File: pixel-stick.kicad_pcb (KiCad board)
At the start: 2 copper layers, 16.5 x 37.1 mm, 16 parts, among them J2 WS28**, U1 AZ1117-3.3, U2 ESP-01v090, U3 SN74LVC1T45DBV, U4 RT9361A

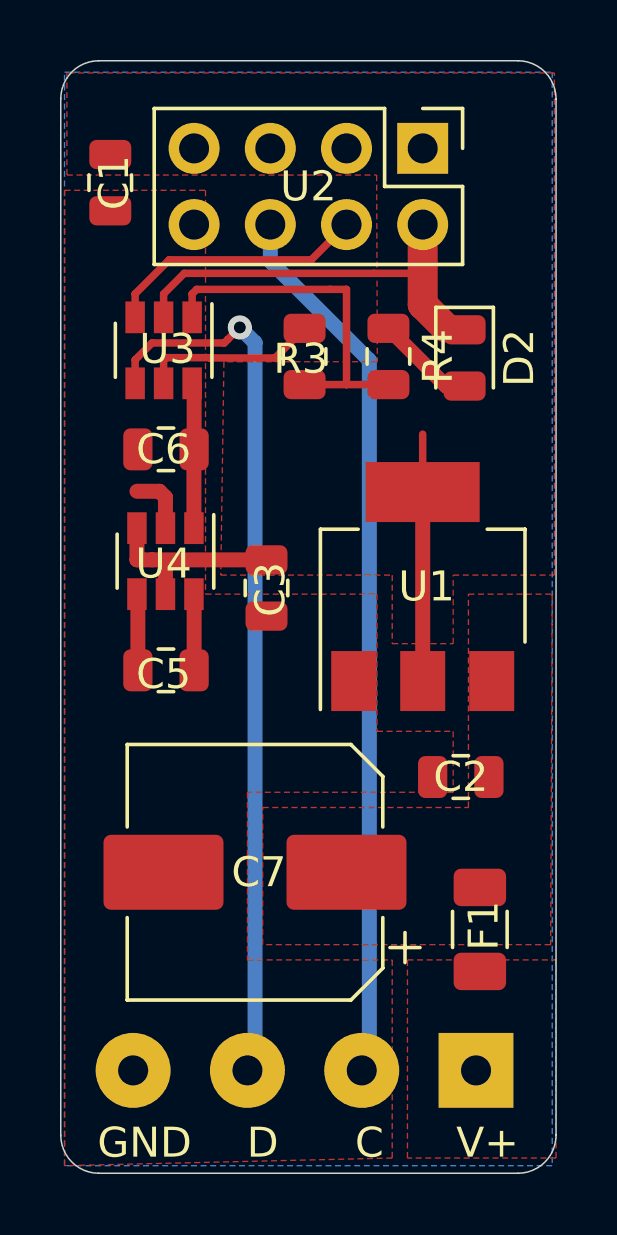
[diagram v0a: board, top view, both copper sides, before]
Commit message: fix drc errors
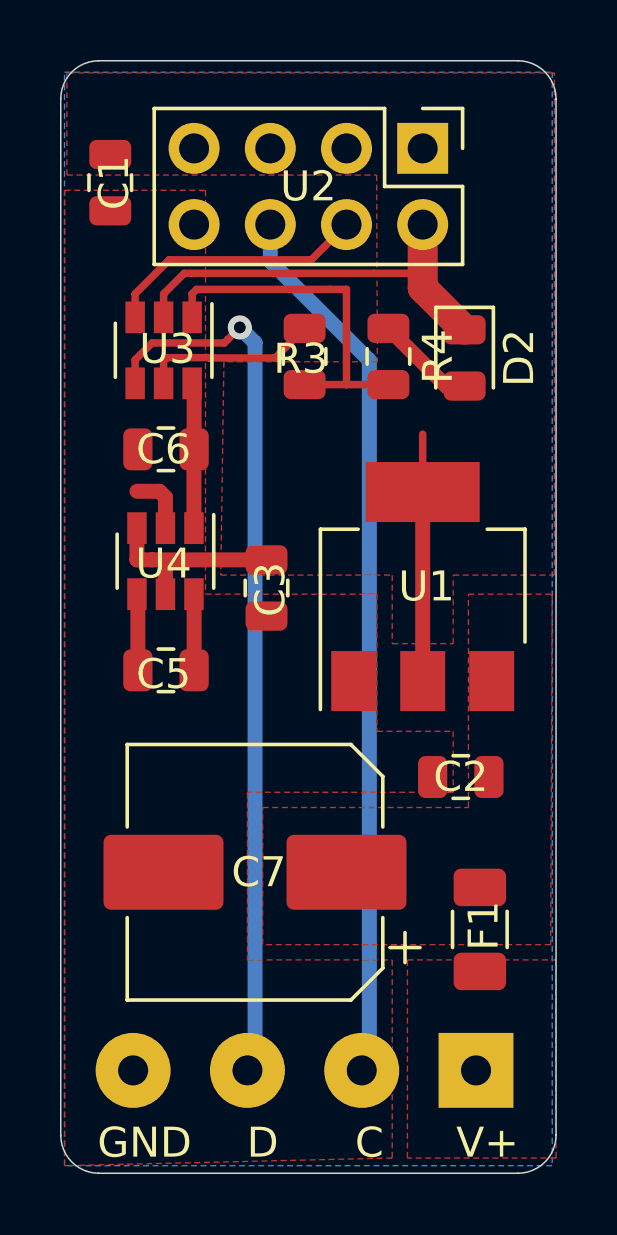
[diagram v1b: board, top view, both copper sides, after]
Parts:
- R4: value 10k -> 120
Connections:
- J2 pad 2: /DATA -> /CLOCK
- J2 pad 3: /CLOCK -> /DATA
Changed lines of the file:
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@@
   )
   (setup
-    (last_trace_width 0.25)
+    (last_trace_width 1)
     (user_trace_width 0.5)
     (user_trace_width 1)
@@
       (effects (font (size 1 1) (thickness 0.15)))
     )
-    (fp_text value 10k (at 0 1.65 90) (layer F.Fab)
+    (fp_text value 120 (at 0 1.65 90) (layer F.Fab)
       (effects (font (size 1 1) (thickness 0.15)))
     )
@@
       (net 1 GND))
     (pad 3 thru_hole circle (at 7.62 0 180) (size 2.49936 2.49936) (drill 1.00076) (layers *.Cu *.Mask)
+      (net 11 /DATA))
+    (pad 2 thru_hole circle (at 3.81 0 180) (size 2.49936 2.49936) (drill 1.00076) (layers *.Cu *.Mask)
       (net 10 /CLOCK))
-    (pad 2 thru_hole circle (at 3.81 0 180) (size 2.49936 2.49936) (drill 1.00076) (layers *.Cu *.Mask)
-      (net 11 /DATA))
     (pad 1 thru_hole rect (at 0 0 180) (size 2.49936 2.49936) (drill 1.00076) (layers *.Cu *.Mask)
       (net 8 /VIN))
@@
   (segment (start 54.460011 60.680011) (end 54.61 60.83) (width 0.25) (layer F.Cu) (net 1))
   (segment (start 52.984989 60.680011) (end 54.460011 60.680011) (width 0.25) (layer F.Cu) (net 1))
-  (segment (start 54.61 61.722) (end 55.372 62.484) (width 1) (layer F.Cu) (net 1))
-  (segment (start 54.61 59.055) (end 54.61 61.722) (width 1) (layer F.Cu) (net 1))
+  (segment (start 54.61 61.1655) (end 56.007 62.5625) (width 1) (layer F.Cu) (net 1))
+  (segment (start 54.61 59.055) (end 54.61 61.1655) (width 1) (layer F.Cu) (net 1))
   (segment (start 52.04 56.485) (end 52.07 56.515) (width 0.25) (layer B.Cu) (net 2))
   (segment (start 54.61 74.27) (end 54.61 67.97) (width 0.5) (layer F.Cu) (net 2))
